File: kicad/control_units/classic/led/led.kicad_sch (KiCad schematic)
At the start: 43 parts, among them J2 Conn_01x05, Q1 BC547, Q2 BC547, Q3 BC547, Q4 BC547, Q5 BC547, Q6 BC547, Q7 BC547, Q8 BC547, U1 74HC595

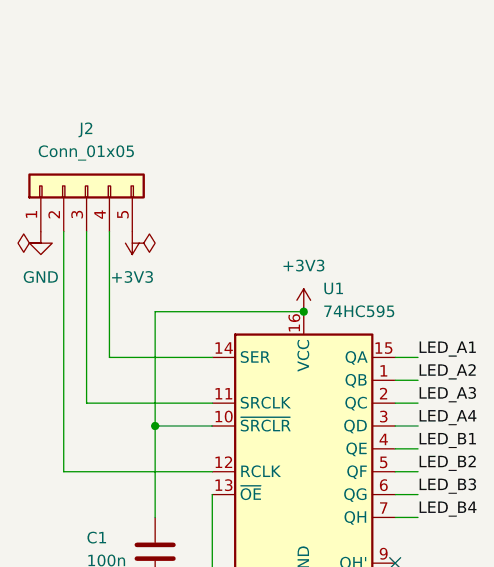
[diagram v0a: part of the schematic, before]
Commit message: feat: Should now be able to order some prototype PCBs to see if this whole thing actually works; note to self, buy some DIP sockets
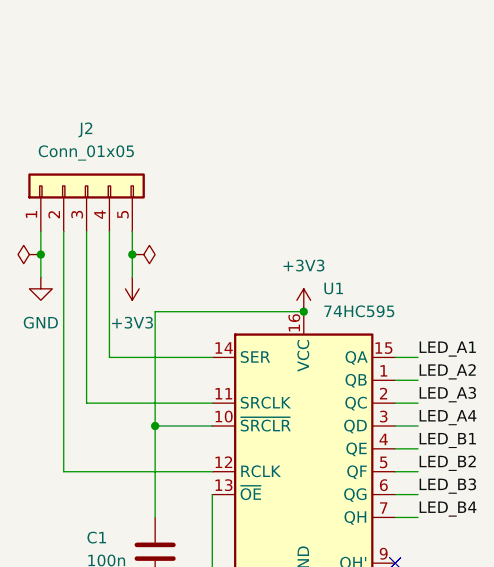
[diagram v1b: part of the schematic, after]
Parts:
- C1: footprint (none) -> Capacitor_THT:C_Disc_D5.0mm_W2.5mm_P2.50mm
- D1, D2, D3, D4, D5, D6, D7, D8: footprint (none) -> LED_THT:LED_D5.0mm
- J2: footprint (none) -> Connector_PinSocket_2.54mm:PinSocket_1x05_P2.54mm_Vertical
- R1, R10, R11, R12, R13, R14, R15, R16, R17, R18, R19, R2, R20, R21, R22, R23, R24, R3, R4, R5, R6, R7, R8, R9: footprint (none) -> Resistor_THT:R_Axial_DIN0207_L6.3mm_D2.5mm_P7.62mm_Horizontal
- U1: footprint (none) -> Package_DIP:DIP-16_W7.62mm
